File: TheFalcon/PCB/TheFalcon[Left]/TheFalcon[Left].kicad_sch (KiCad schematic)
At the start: 36 parts, among them J1 Conn_01x04_Pin, J2 Conn_02x05_Odd_Even, J3 Conn_01x04_Pin, SW1 SW_Push, SW2 SW_Push, SW3 SW_SPDT, U1 STM32F103CBTx, U2 USBLC6-2P6, U3 USBLC6-2P6, U4 AMS1117-3.3, U5 USBLC6-2P6, Y1 X322516MOB4SI

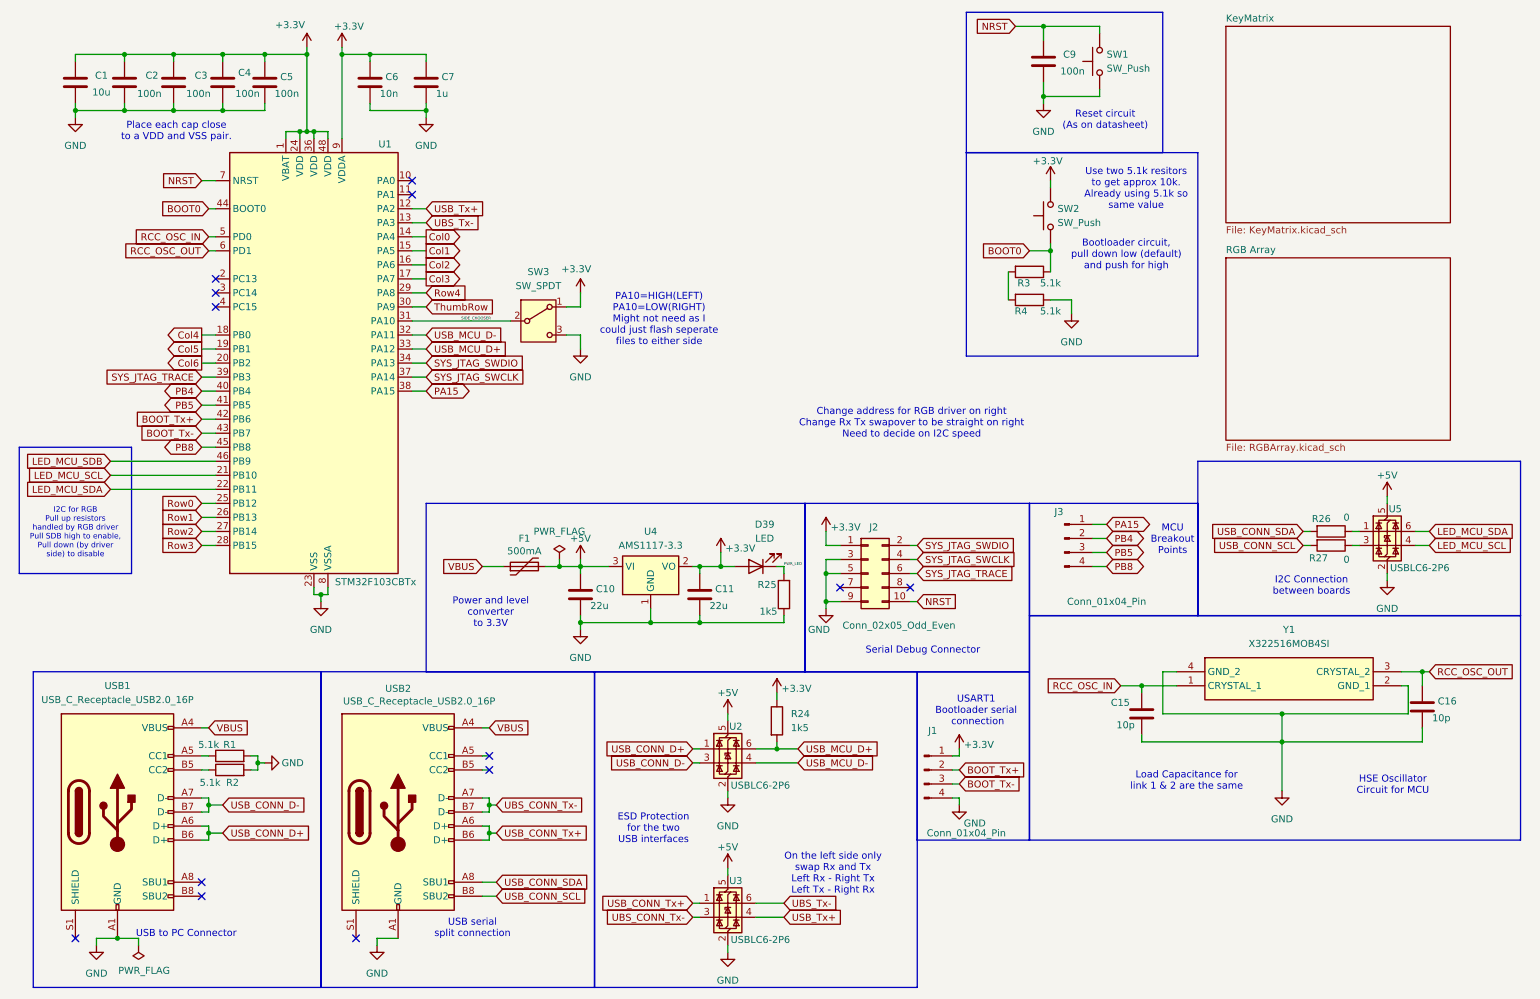
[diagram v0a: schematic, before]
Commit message: Save
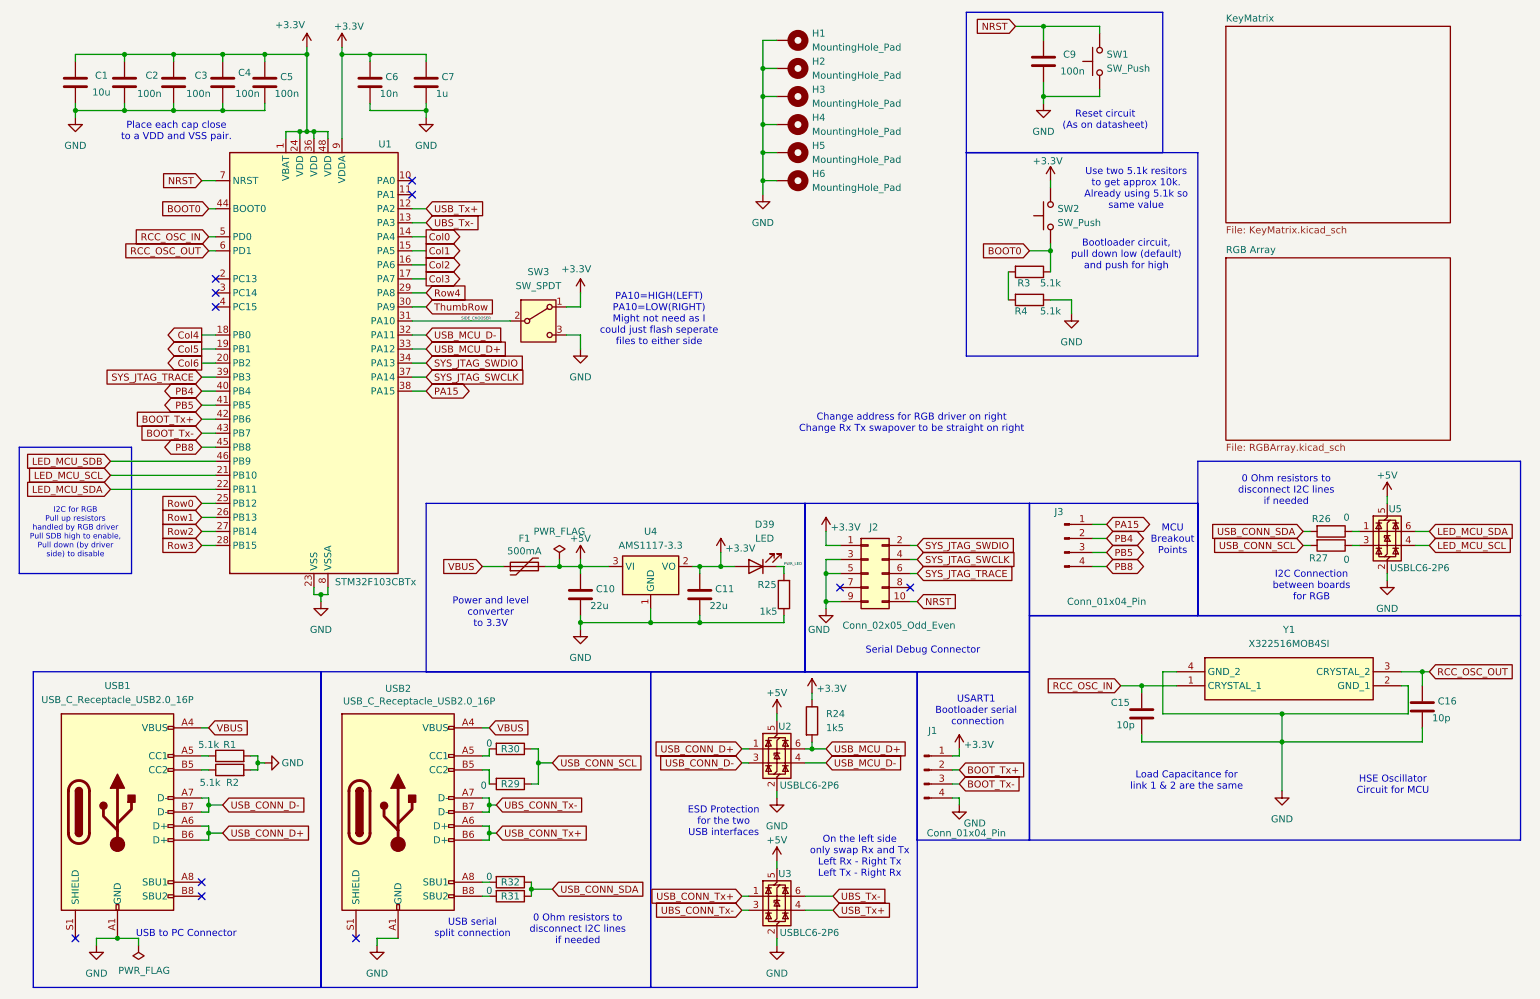
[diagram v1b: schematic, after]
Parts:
- added H1, H2, H3, H4, H5, H6: MountingHole_Pad, MountingHole:MountingHole_3.2mm_M3_Pad_Via, symbol Mechanical:MountingHole_Pad
- added R29, R30, R31, R32: 0, Resistor_SMD:R_0805_2012Metric, symbol Device:R
- R1, R2, R3, R4: footprint (none) -> Resistor_SMD:R_0603_1608Metric
- R24, R25: footprint (none) -> Resistor_SMD:R_0201_0603Metric
- R26, R27: footprint (none) -> Resistor_SMD:R_0805_2012Metric
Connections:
- net GND: now also H1.1, H2.1, H3.1, H4.1, H5.1, H6.1
- net USB_CONN_SCL: now also R29.1, R30.1; no longer USB2.B8 (SBU2)
- net USB_CONN_SDA: now also R31.1, R32.1; no longer USB2.A8 (SBU1)
- net at USB2.A5 (CC1): now also R30.2
- net at USB2.B5 (CC2): now also R29.2
- new net: R32.2, USB2.A8 (SBU1)
- new net: R31.2, USB2.B8 (SBU2)
- no-connect marks 13 -> 11
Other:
- note added: "0 Ohm resistors to disconnect I2C lines if needed"
- note added: "Change address for RGB driver on right Change Rx Tx swapover to be straight on right"
- note added: "I2C Connection between boards for RGB"
- note removed: "Change address for RGB driver on right Change Rx Tx swapover to be straight on right Need to decide on I2C speed"
- note removed: "I2C Connection between boards"
- moved on the sheet: R24, U2, U3

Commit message: save
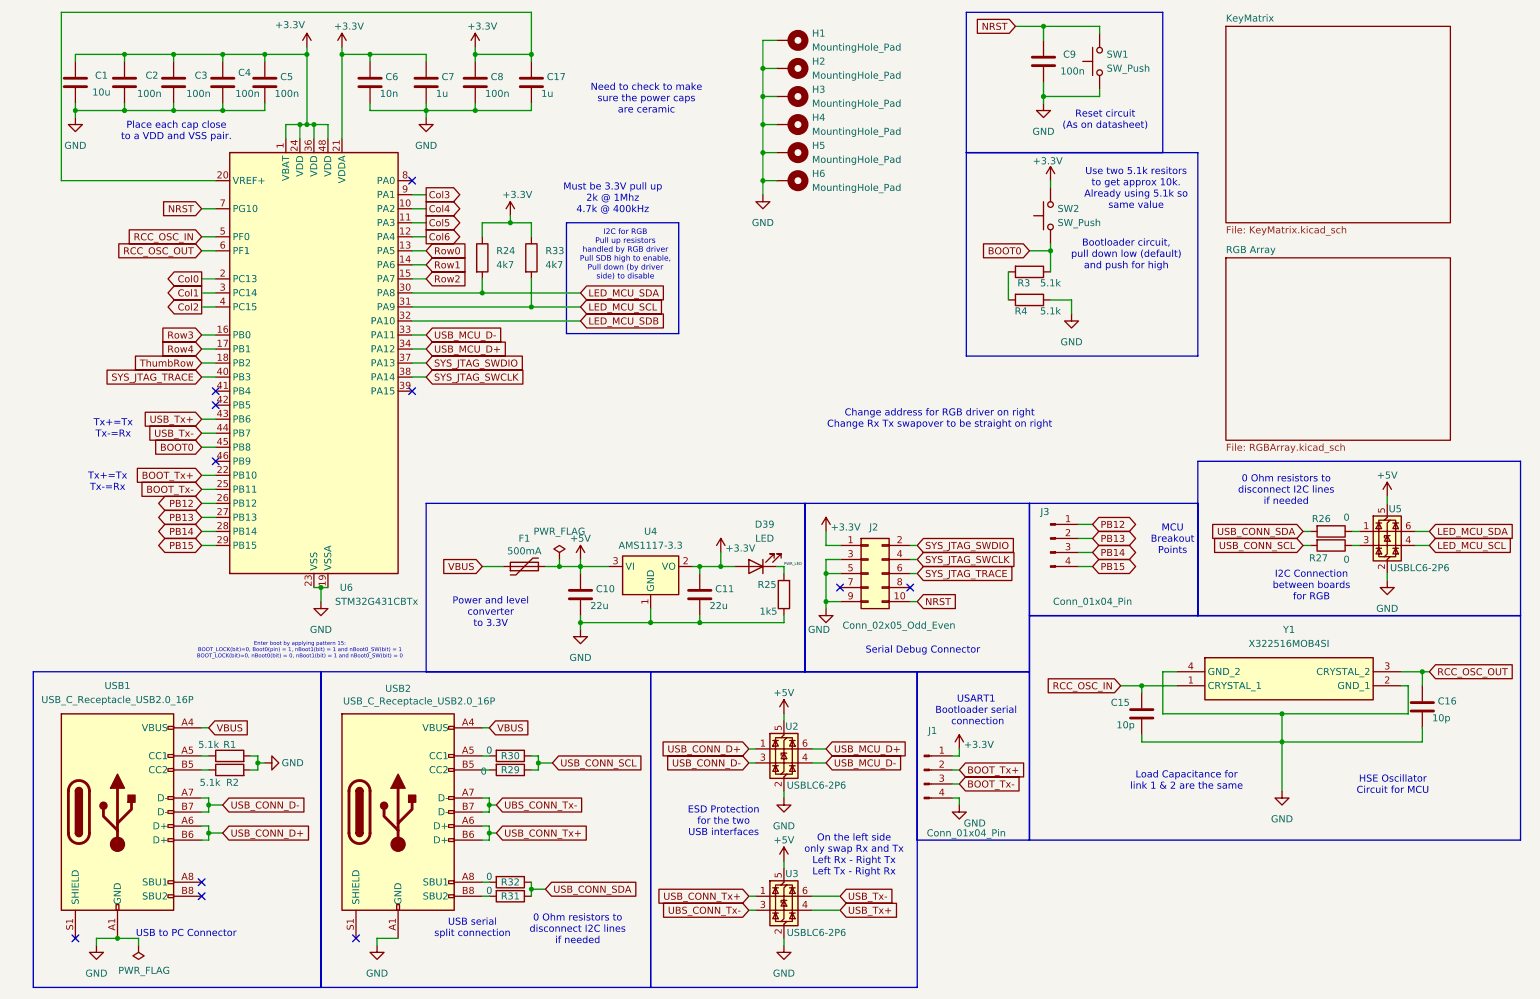
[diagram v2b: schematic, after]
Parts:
- removed SW3: SW_SPDT, symbol Switch:SW_SPDT
- removed U1: STM32F103CBTx, Package_QFP:LQFP-48_7x7mm_P0.5mm, symbol MCU_ST_STM32F1:STM32F103CBTx
- added C17: 1u, Capacitor_SMD:C_0603_1608Metric, symbol Device:C
- added C8: 100n, Capacitor_SMD:C_0603_1608Metric, symbol Device:C
- added R33: 4k7, Resistor_SMD:R_0201_0603Metric, symbol Device:R
- added U6: STM32G431CBTx, Package_QFP:LQFP-48_7x7mm_P0.5mm, symbol MCU_ST_STM32G4:STM32G431CBTx
- D39: footprint (none) -> LED_SMD:LED_0805_2012Metric
- R24: value 1k5 -> 4k7
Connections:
- net +3.3V: now also C17.1, C8.1, R33.1, U6.1 (VBAT), U6.20 (VREF+), U6.21 (VDDA), U6.24 (VDD), U6.36 (VDD), U6.48 (VDD)
- net BOOT0: now also U6.45 (PB8)
- net BOOT_Tx+: now also U6.22 (PB10)
- net BOOT_Tx-: now also U6.25 (PB11)
- net Col0: now also U6.2 (PC13)
- net Col1: now also U6.3 (PC14)
- net Col2: now also U6.4 (PC15)
- net Col3: now also U6.9 (PA1)
- net Col4: now also U6.10 (PA2)
- net Col5: now also U6.11 (PA3)
- net Col6: now also U6.12 (PA4)
- net GND: now also C17.2, C8.2, U6.19 (VSSA), U6.23 (VSS), U6.35 (VSS), U6.47 (VSS)
- net LED_MCU_SCL: now also R33.2, U6.31 (PA9)
- net LED_MCU_SDA: now also R24.2, U6.30 (PA8)
- net LED_MCU_SDB: now also U6.32 (PA10)
- net NRST: now also U6.7 (PG10)
- net RCC_OSC_IN: now also U6.5 (PF0)
- net RCC_OSC_OUT: now also U6.6 (PF1)
- net Row0: now also U6.13 (PA5)
- net Row1: now also U6.14 (PA6)
- net Row2: now also U6.15 (PA7)
- net Row3: now also U6.16 (PB0)
- net Row4: now also U6.17 (PB1)
- net SYS_JTAG_SWCLK: now also U6.38 (PA14)
- net SYS_JTAG_SWDIO: now also U6.37 (PA13)
- net SYS_JTAG_TRACE: now also U6.40 (PB3)
- net ThumbRow: now also U6.18 (PB2)
- net USB_MCU_D+: now also U6.34 (PA12); no longer R24.2
- net USB_MCU_D-: now also U6.33 (PA11)
- net USB_Tx+: now also U6.43 (PB6)
- net PA15 renamed PB12
- net PB12: now also U6.26 (PB12)
- net PB4 renamed PB13
- net PB13: now also U6.27 (PB13)
- net PB5 renamed PB14
- net PB14: now also U6.28 (PB14)
- net PB8 renamed PB15
- net PB15: now also U6.29 (PB15)
- net UBS_Tx- renamed USB_Tx-
- net USB_Tx-: now also U6.44 (PB7)
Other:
- note added: "Enter boot by applying pattern 15: BOOT_LOCK(bit)=0, Boot0(pin) = 1, nBoot1(bit) = 1 and nBoot0_SW(bit) = 1 BOOT_LOCK(bit)=0, nBoot0(bit) = 0, nBoot1(bit) = 1 and nBoot0_SW(bit) = 0"
- note added: "Must be 3.3V pull up 2k @ 1Mhz 4.7k @ 400kHz"
- note added: "Need to check to make sure the power caps are ceramic"
- note added: "Tx+=Tx Tx-=Rx"
- note removed: "PA10=HIGH(LEFT) PA10=LOW(RIGHT) Might not need as I could just flash seperate files to either side"
- moved on the sheet: J3, R29, R30, U2, U3

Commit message: save
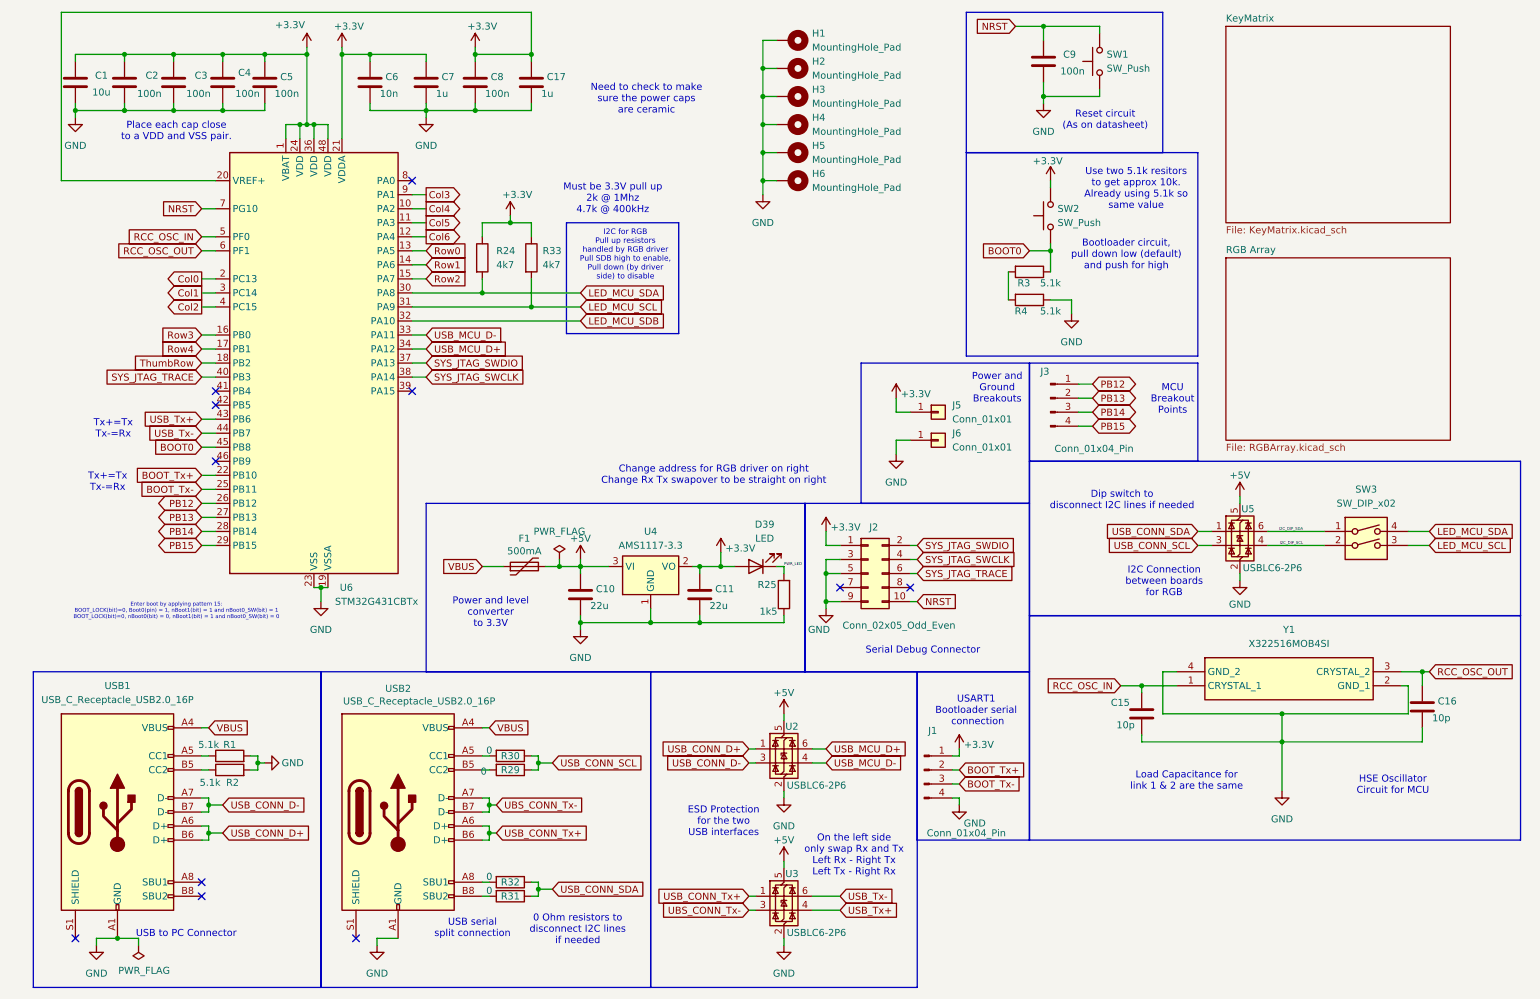
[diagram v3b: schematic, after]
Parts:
- removed R26, R27: 0, Resistor_SMD:R_0805_2012Metric, symbol Device:R
- added J5, J6: Conn_01x01, Connector_Wire:SolderWire-0.1sqmm_1x01_D0.4mm_OD1mm, symbol Connector_Generic:Conn_01x01
- added SW3: SW_DIP_x02, Button_Switch_SMD:SW_DIP_SPSTx02_Slide_KingTek_DSHP02TS_W7.62mm_P1.27mm, symbol Switch:SW_DIP_x02
- F1: footprint (none) -> Fuse:Fuse_1206_3216Metric
- J1, J3: footprint (none) -> Connector_PinSocket_2.54mm:PinSocket_1x04_P2.54mm_Vertical
- J2: footprint (none) -> Connector_PinSocket_2.54mm:PinSocket_2x05_P2.54mm_Vertical
- SW1, SW2: footprint (none) -> Button_Switch_SMD:SW_SPST_B3U-1000P
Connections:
- net +3.3V: now also J5.1 (Pin_1)
- net GND: now also J6.1 (Pin_1)
- net LED_MCU_SCL: now also SW3.3; no longer U5.4 (I/O2)
- net LED_MCU_SDA: now also SW3.4; no longer U5.6 (I/O1)
- net USB_CONN_SCL: now also U5.3 (I/O2)
- net USB_CONN_SDA: now also U5.1 (I/O1)
- new net I2C_DIP_SCL: SW3.2, U5.4 (I/O2)
- new net I2C_DIP_SDA: SW3.1, U5.6 (I/O1)
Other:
- note added: "Dip switch to disconnect I2C lines if needed"
- note added: "Power and Ground Breakouts"
- moved on the sheet: J3, U5
